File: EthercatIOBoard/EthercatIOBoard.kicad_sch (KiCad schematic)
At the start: 5 parts, among them J1 Conn_01x03

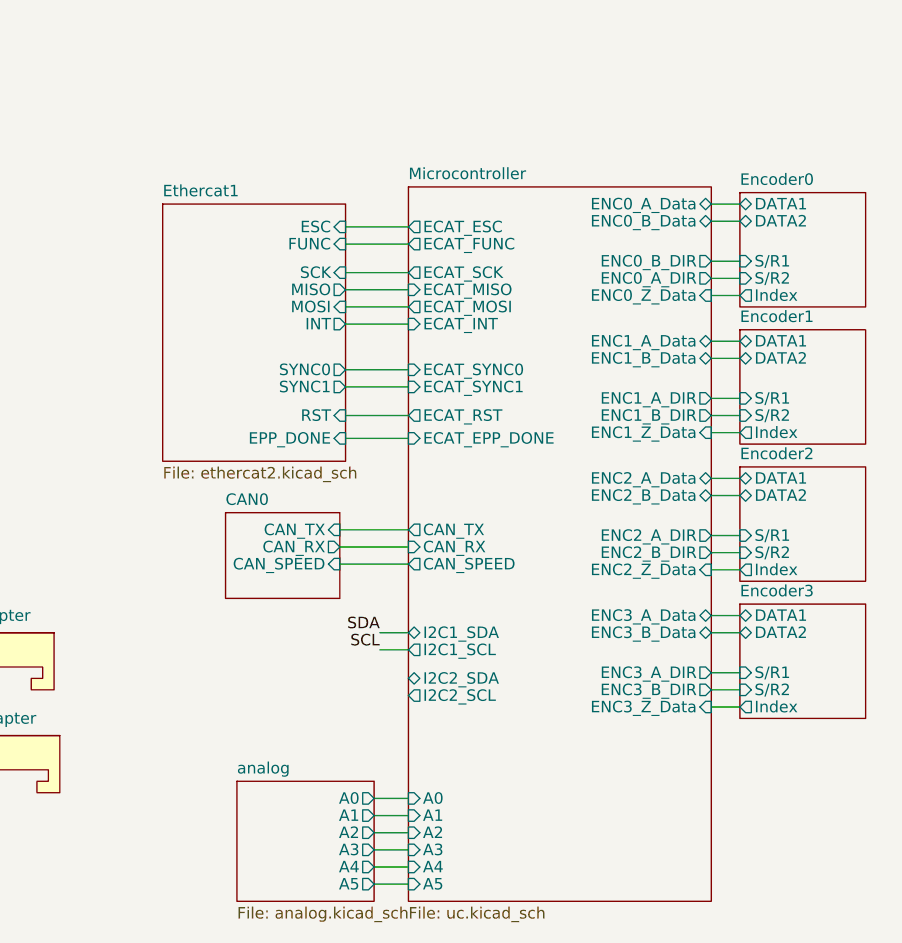
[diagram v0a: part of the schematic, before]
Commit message: some cleanup
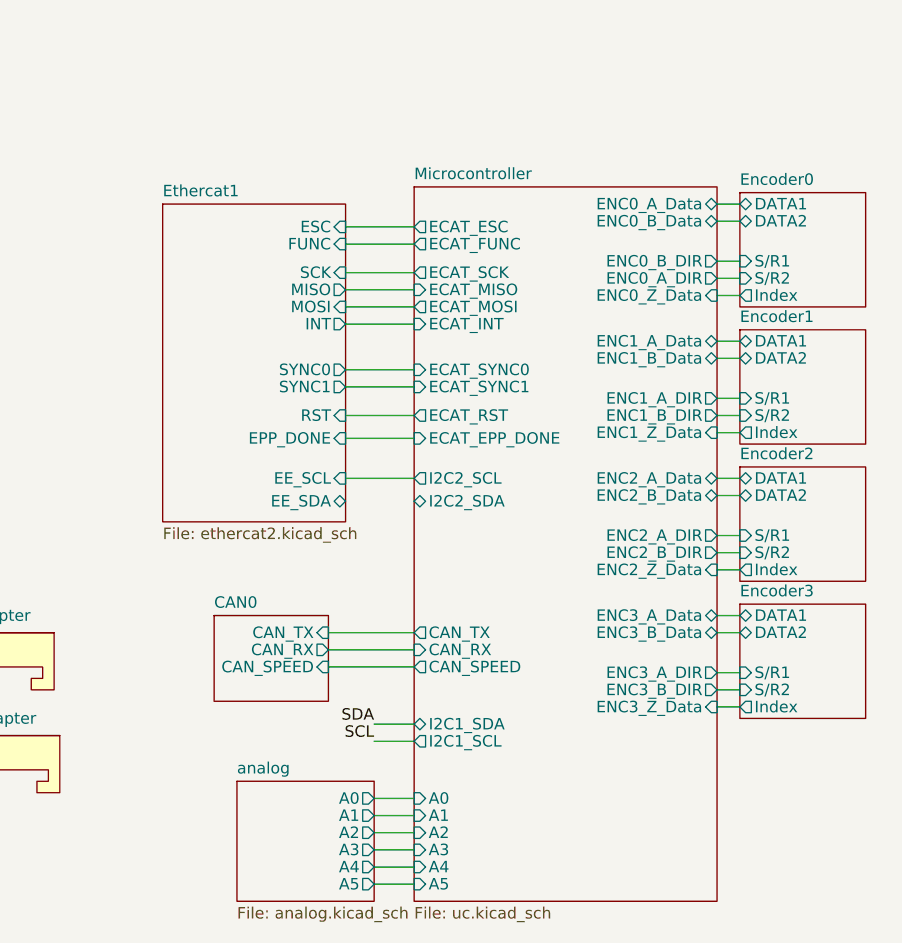
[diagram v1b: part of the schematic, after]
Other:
- sheet Ethercat1 ports: added EE_SCL, EE_SDA; removed none
